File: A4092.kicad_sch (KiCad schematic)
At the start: 0 parts

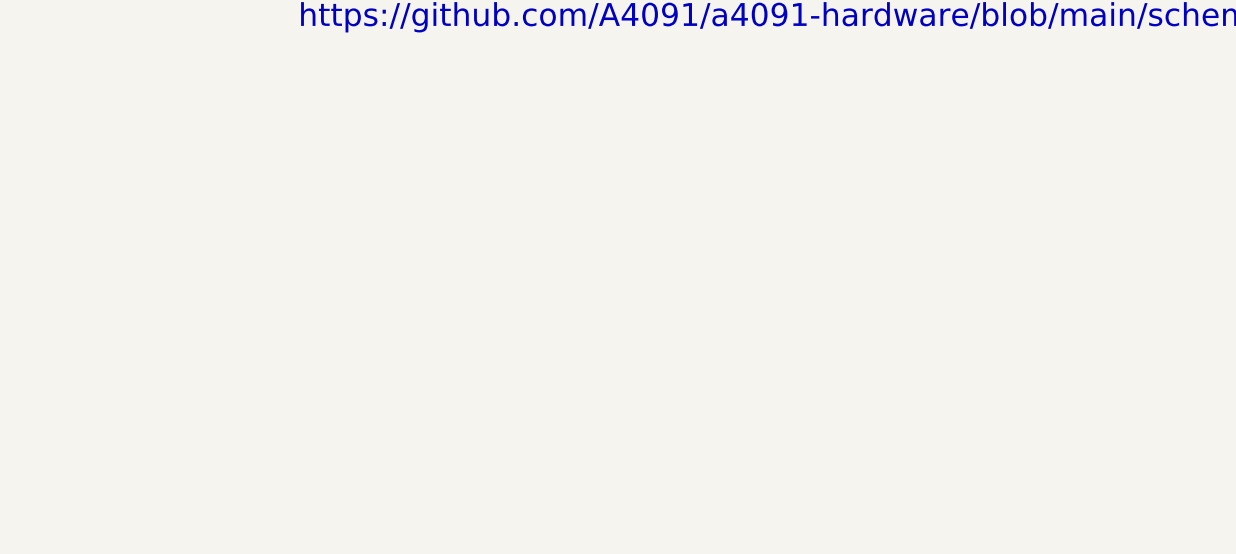
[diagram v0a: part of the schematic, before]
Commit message: Update design
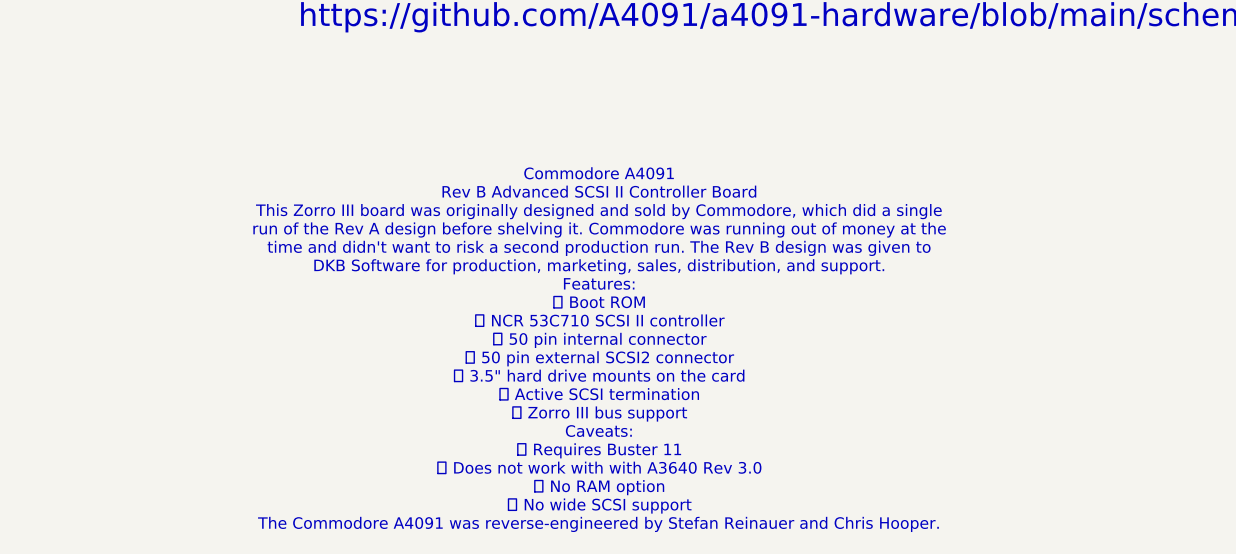
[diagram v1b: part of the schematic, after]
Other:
- note added: "Commodore A4091 Rev B Advanced SCSI II Controller Board This Zorro III board was originally designed and sold by Commodore, which did a single run of the Rev A design before shelving it. Commodore was running out of money at the time and didn't want to risk a second production run. The Rev B design was given to DKB Software for production, marketing, sales, distribution, and support. Features: 􂀢 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"
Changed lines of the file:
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@@
 	(generator_version "9.0")
 	(paper "A4")
+	(text "Commodore A4091\nRev B Advanced SCSI II Controller Board\nThis Zorro III board was originally designed and sold by Commodore, which did a single\nrun of the Rev A design before shelving it. Commodore was running out of money at the\ntime and didn't want to risk a second production run. The Rev B design was given to\nDKB Software for production, marketing, sales, distribution, and support.\nFeatures:\n􂀢 Boot ROM\n􂀢 NCR 53C710 SCSI II controller\n􂀢 50 pin internal connector\n􂀢 50 pin external SCSI2 connector\n􂀢 3.5\" hard drive mounts on the card\n􂀢 Active SCSI termination\n􂀢 Zorro III bus support\nCaveats:\n􂀢 Requires Buster 11\n􂀢 Does not work with with A3640 Rev 3.0\n􂀢 No RAM option\n􂀢 No wide SCSI support\nThe Commodore A4091 was reverse-engineered by Stefan Reinauer and Chris Hooper."
+		(exclude_from_sim no)
+		(at 89.916 155.448 0)
+		(effects
+			(font
+				(size 1.27 1.27)
+			)
+		)
+	)
 	(text "GitHub Project:\nhttps://github.com/A4091/\n\nSchematics:\nhttps://github.com/A4091/a4091-hardware/blob/main/schematics/ReA4091_Rev4_2023-05-15_Schematic.pdf"
 		(exclude_from_sim no)
